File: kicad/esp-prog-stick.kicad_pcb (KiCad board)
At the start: 4 copper layers, 15 x 35 mm, 15 parts, among them J1 USB_A, J2 JST SM06B-SHLS-TF, Q1 S8050, Q2 S8050, U1 AZ1117-3.3, U2 CH340G, Y1 CSTNE12M0G550000R0

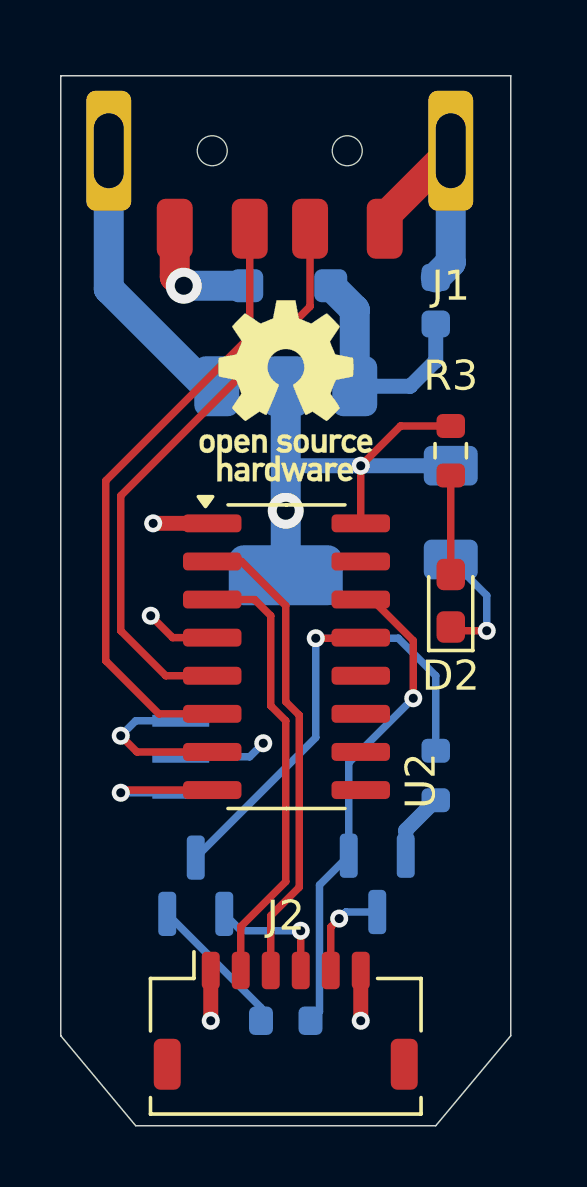
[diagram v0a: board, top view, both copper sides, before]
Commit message: Revision 2
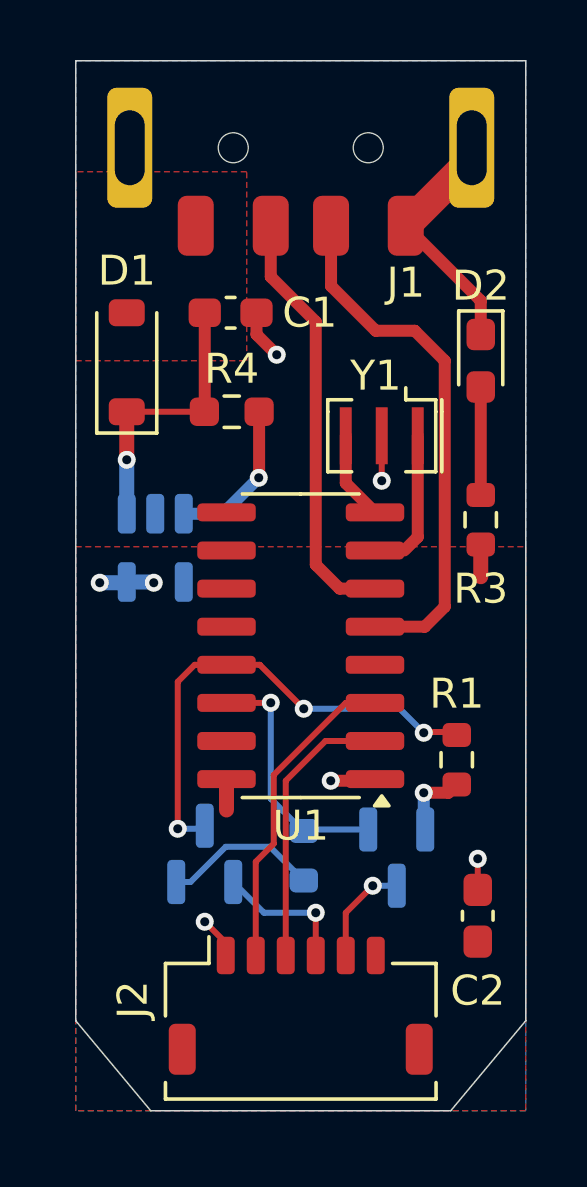
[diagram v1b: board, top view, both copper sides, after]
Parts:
- removed REF**: OSHW-Logo_5.7x6mm_SilkScreen, Symbol:OSHW-Logo_5.7x6mm_SilkScreen
- added R4: 39K, Resistor_SMD:R_0603_1608Metric_Pad0.98x0.95mm_HandSolder, F.Cu at (198.2, 66.7)
- C1: value 10uF -> 1uF; footprint Capacitor_SMD:C_0603_1608Metric -> Capacitor_SMD:C_0603_1608Metric_Pad1.08x0.95mm_HandSolder; moved to F.Cu
- C2: value 22uF -> 1uF; footprint Capacitor_SMD:C_1206_3216Metric_Pad1.33x1.80mm_HandSolder -> Capacitor_SMD:C_0603_1608Metric_Pad1.08x0.95mm_HandSolder; moved to F.Cu
- D1: value DSL16 -> PMEG4030; footprint Diode_SMD:D_SOD-123F -> Diode_SMD:D_SOD-123; moved to F.Cu
- R1, Y1: moved to F.Cu
- R3: value 2K2 -> 100R
- U1: value AZ1117-3.3 -> CH340G; footprint Package_TO_SOT_SMD:SOT-223-3_TabPin2 -> Package_SO:SOIC-16_3.9x9.9mm_P1.27mm; moved to F.Cu
- U2: value CH340G -> TLV75533PDBV; footprint Package_SO:SOIC-16_3.9x9.9mm_P1.27mm -> Package_TO_SOT_SMD:SOT-23-5; moved to B.Cu
- moved C2 13.5 mm to (206.4, 83.5)
- moved Y1 12.6 mm to (203.2, 67.5), turned to 180 degrees
- moved D2 8.06 mm to (206.5, 65.0), turned to -90 degrees
- moved C1 6.85 mm to (198.2, 63.4), turned to 180 degrees
- moved D1 5.97 mm to (194.7, 65.0), turned to 90 degrees
- moved U2 5.68 mm to (195.7, 71.2), turned to -90 degrees
- moved R2 5.53 mm to (200.6, 81.5), turned to -90 degrees
- moved U1 5.52 mm to (200.5, 74.5), turned to 180 degrees
- moved R3 2.51 mm to (206.5, 70.3), turned to 90 degrees
- moved Q2 1.10 mm to (197.3, 81.4)
- moved Q1 1.09 mm to (203.7, 81.6)
- moved R1 0.87 mm to (205.7, 78.3)
- moved J2 0.71 mm to (200.5, 86.5)
- moved J1 0.71 mm to (199.5, 60.5)
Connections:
- net /ESP_EN renamed /Schematics/ESP_EN
- net /ESP_IO0 renamed /Schematics/BOOT
- C1 pad 1: +5V -> GND
- C1 pad 2: GND -> +5V
- C2 pad 1: +3V3 -> GND
- C2 pad 2: GND -> +3V3
- J1 pad 2: /USB_D- -> /Schematics/USB_D-
- J1 pad 3: /USB_D+ -> /Schematics/USB_D+
- J2 pad 2: /RX -> /Schematics/RX
- J2 pad 3: /TX -> /Schematics/TX
- Q1 pad 1: /RTS -> /Schematics/RTS
- Q2 pad 3: /DTR -> /Schematics/DTR
- R1 pad 1: /DTR -> /Schematics/DTR
- R2 pad 1: /RTS -> /Schematics/RTS
- U1 pad 2: +3V3 -> /Schematics/TX
- U1 pad 3: +5V -> /Schematics/RX
- U2 pad 1: GND -> +5V
- U2 pad 2: /TX -> GND
- U2 pad 3: /RX -> Net-(U2-EN)
- U2 pad 4: +3V3 -> unconnected-(U2-NC-Pad4)
- U2 pad 5: /USB_D+ -> +3V3
- Y1 pad 1: Net-(U2-XI) -> Net-(U1-XI)
- Y1 pad 3: Net-(U2-XO) -> Net-(U1-XO)
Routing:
- net /USB_D-: track 20.7 -> 0.00 mm
- net /USB_D+: track 19.7 -> 0.00 mm
- net +3V3: track 22.8 -> 3.93 mm, vias 4 -> 2
- net /Schematics/USB_D+: track 0.00 -> 17.6 mm
- net /DTR: track 17.5 -> 0.00 mm, vias 1 -> 0
- net /Schematics/DTR: track 0.00 -> 16.4 mm, vias 0 -> 3
- net /RTS: track 16.4 -> 0.00 mm, vias 1 -> 0
- net /TX: track 15.8 -> 0.00 mm
- net /RX: track 14.8 -> 0.00 mm
- net /Schematics/USB_D-: track 0.00 -> 14.2 mm
- net GND: track 28.2 -> 15.3 mm, vias 4 -> 5
- net /Schematics/RX: track 0.00 -> 10.6 mm
- net /Schematics/TX: track 0.00 -> 9.35 mm
- net /Schematics/RTS: track 0.00 -> 8.35 mm, vias 0 -> 1
- net Net-(U2-XI): track 5.48 -> 0.00 mm, vias 1 -> 0
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- added copper zone on F.Cu, net +3V3
- added copper zone on B.Cu, net GND
- added copper zone on F.Cu, net Net-(D1-A)
- removed copper zone on In1.Cu, net +3V3
- removed copper zone on In2.Cu, net GND
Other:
- copper layers 4 -> 2
- board text removed: "github.com/harexew/esp-prog-stick"
